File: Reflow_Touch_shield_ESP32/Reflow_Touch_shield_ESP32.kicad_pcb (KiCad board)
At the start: 2 copper layers, 88.5 x 52.5 mm, 3 parts, among them IC1 MAX6675, J1 Conn_01x14

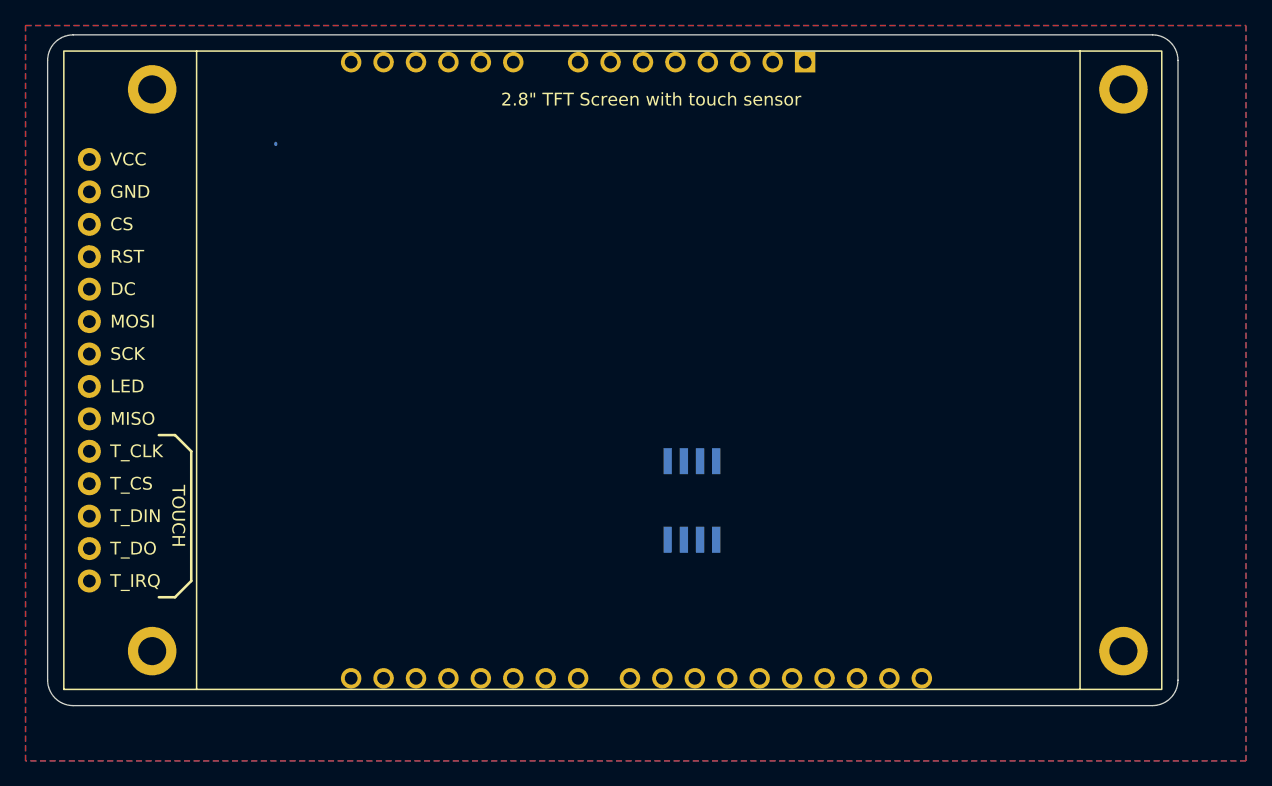
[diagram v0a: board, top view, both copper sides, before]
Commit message: Update PCB
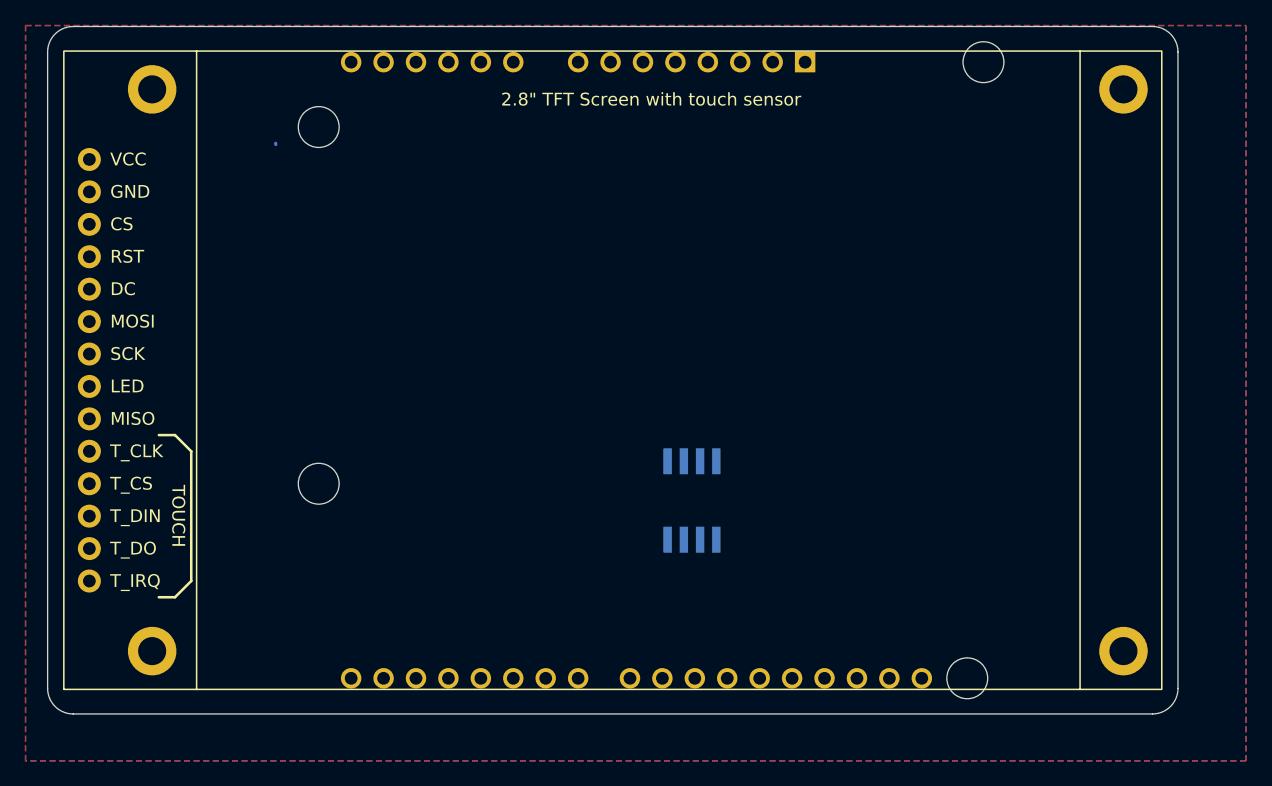
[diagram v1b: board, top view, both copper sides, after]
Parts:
- A1: footprint Module:Arduino_UNO_R3 -> Module:Arduino_UNO_R3_WithMountingHoles
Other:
- board size 88.5 x 52.5 mm -> 88.5 x 53.8 mm
